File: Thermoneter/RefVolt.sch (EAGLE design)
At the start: 4 parts, among them IC1 OP-AMP-1TSV521ICT

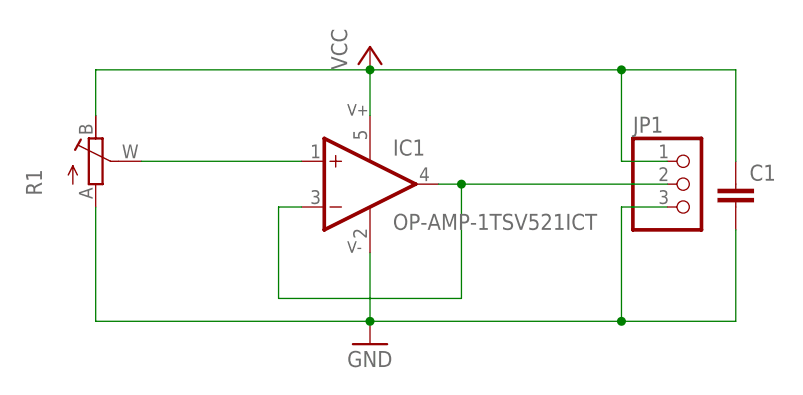
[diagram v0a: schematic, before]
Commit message: _Something
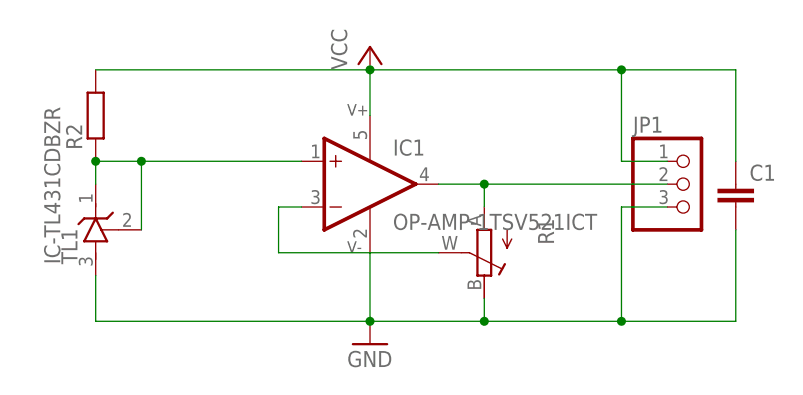
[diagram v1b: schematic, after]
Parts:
- added R2: (no value), Namenlos:R_0805
- added TL1: IC-TL431CDBZR, Namenlos:IC-TL431CDBZR
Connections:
- new net N$7: IC1G$1.+IN, R2.1, TL1.C, TL1.R
- net GND: now also R1.E, TL1.A; no longer R1.A
- net N$1: now also R1.S; no longer IC1G$1.OUT, JP1.2
- net N$4: now also IC1G$1.OUT, JP1.2, R1.A; no longer IC1G$1.+IN, R1.S
- net VCC: now also R2.2; no longer R1.E
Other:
- moved on the sheet: R1
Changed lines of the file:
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@@
 <?xml version="1.0" encoding="utf-8"?>
 <!DOCTYPE eagle SYSTEM "eagle.dtd">
-<eagle version="8.0.0">
+<eagle version="8.0.1">
 <drawing>
 <settings>
@@
 <part name="GND1" library="supply1" deviceset="GND" device=""/>
 <part name="P+1" library="supply1" deviceset="VCC" device=""/>
+<part name="TL1" library="Namenlos" deviceset="IC-TL431" device="CDBZR"/>
+<part name="R2" library="Namenlos" deviceset="R_" device="0805"/>
 </parts>
 <sheets>
@@
 <instances>
 <instance part="IC1" gate="G$1" x="30.48" y="33.02"/>
-<instance part="R1" gate="G$1" x="0" y="35.56"/>
+<instance part="R1" gate="G$1" x="43.18" y="25.4" rot="R180"/>
 <instance part="IC1" gate="G$2" x="30.48" y="33.02"/>
 <instance part="JP1" gate="A" x="66.04" y="33.02"/>
@@
 <instance part="GND1" gate="1" x="30.48" y="15.24"/>
 <instance part="P+1" gate="VCC" x="30.48" y="48.26"/>
+<instance part="TL1" gate="G$1" x="0" y="27.94" rot="MR90"/>
+<instance part="R2" gate="G$1" x="0" y="40.64" rot="R90"/>
 </instances>
 <busses>
@@
 <pinref part="IC1" gate="G$1" pin="-IN"/>
 <wire x1="22.86" y1="30.48" x2="20.32" y2="30.48" width="0.1524" layer="91"/>
-<wire x1="20.32" y1="30.48" x2="20.32" y2="20.32" width="0.1524" layer="91"/>
-<wire x1="20.32" y1="20.32" x2="40.64" y2="20.32" width="0.1524" layer="91"/>
-<wire x1="40.64" y1="20.32" x2="40.64" y2="33.02" width="0.1524" layer="91"/>
-<pinref part="IC1" gate="G$1" pin="OUT"/>
-<wire x1="40.64" y1="33.02" x2="38.1" y2="33.02" width="0.1524" layer="91"/>
-<pinref part="JP1" gate="A" pin="2"/>
-<wire x1="63.5" y1="33.02" x2="40.64" y2="33.02" width="0.1524" layer="91"/>
-<junction x="40.64" y="33.02"/>
-</segment>
-</net>
-<net name="N$4" class="0">
-<segment>
 <pinref part="R1" gate="G$1" pin="S"/>
-<pinref part="IC1" gate="G$1" pin="+IN"/>
-<wire x1="5.08" y1="35.56" x2="22.86" y2="35.56" width="0.1524" layer="91"/>
+<wire x1="38.1" y1="25.4" x2="20.32" y2="25.4" width="0.1524" layer="91"/>
+<wire x1="20.32" y1="25.4" x2="20.32" y2="30.48" width="0.1524" layer="91"/>
 </segment>
 </net>
@@
 <pinref part="IC1" gate="G$2" pin="V-"/>
 <wire x1="30.48" y1="25.4" x2="30.48" y2="17.78" width="0.1524" layer="91"/>
-<wire x1="30.48" y1="17.78" x2="58.42" y2="17.78" width="0.1524" layer="91"/>
+<wire x1="30.48" y1="17.78" x2="43.18" y2="17.78" width="0.1524" layer="91"/>
+<wire x1="43.18" y1="17.78" x2="58.42" y2="17.78" width="0.1524" layer="91"/>
 <wire x1="58.42" y1="17.78" x2="58.42" y2="30.48" width="0.1524" layer="91"/>
 <pinref part="JP1" gate="A" pin="3"/>
 <wire x1="58.42" y1="30.48" x2="63.5" y2="30.48" width="0.1524" layer="91"/>
-<pinref part="R1" gate="G$1" pin="A"/>
-<wire x1="0" y1="30.48" x2="0" y2="17.78" width="0.1524" layer="91"/>
 <wire x1="0" y1="17.78" x2="30.48" y2="17.78" width="0.1524" layer="91"/>
 <junction x="30.48" y="17.78"/>
@@
 <junction x="58.42" y="17.78"/>
 <pinref part="GND1" gate="1" pin="GND"/>
+<pinref part="R1" gate="G$1" pin="E"/>
+<wire x1="43.18" y1="20.32" x2="43.18" y2="17.78" width="0.1524" layer="91"/>
+<junction x="43.18" y="17.78"/>
+<pinref part="TL1" gate="G$1" pin="A"/>
+<wire x1="0" y1="22.86" x2="0" y2="17.78" width="0.1524" layer="91"/>
 </segment>
 </net>
@@
 <pinref part="JP1" gate="A" pin="1"/>
 <wire x1="58.42" y1="35.56" x2="63.5" y2="35.56" width="0.1524" layer="91"/>
-<pinref part="R1" gate="G$1" pin="E"/>
-<wire x1="0" y1="40.64" x2="0" y2="45.72" width="0.1524" layer="91"/>
 <wire x1="0" y1="45.72" x2="30.48" y2="45.72" width="0.1524" layer="91"/>
 <junction x="30.48" y="45.72"/>
@@
 <junction x="58.42" y="45.72"/>
 <pinref part="P+1" gate="VCC" pin="VCC"/>
-</segment>
-</net>
+<pinref part="R2" gate="G$1" pin="2"/>
+</segment>
+</net>
+<net name="N$4" class="0">
+<segment>
+<pinref part="R1" gate="G$1" pin="A"/>
+<pinref part="IC1" gate="G$1" pin="OUT"/>
+<wire x1="43.18" y1="30.48" x2="43.18" y2="33.02" width="0.1524" layer="91"/>
+<wire x1="43.18" y1="33.02" x2="38.1" y2="33.02" width="0.1524" layer="91"/>
+<pinref part="JP1" gate="A" pin="2"/>
+<wire x1="63.5" y1="33.02" x2="43.18" y2="33.02" width="0.1524" layer="91"/>
+<junction x="43.18" y="33.02"/>
+</segment>
+</net>
+<net name="N$7" class="0">
+<segment>
+<pinref part="TL1" gate="G$1" pin="C"/>
+<pinref part="R2" gate="G$1" pin="1"/>
+<pinref part="TL1" gate="G$1" pin="R"/>
+<wire x1="5.08" y1="27.94" x2="5.08" y2="35.56" width="0.1524" layer="91"/>
+<wire x1="5.08" y1="35.56" x2="0" y2="35.56" width="0.1524" layer="91"/>
+<junction x="0" y="35.56"/>
+<wire x1="0" y1="35.56" x2="0" y2="33.02" width="0.1524" layer="91"/>
+<pinref part="IC1" gate="G$1" pin="+IN"/>
+<wire x1="22.86" y1="35.56" x2="5.08" y2="35.56" width="0.1524" layer="91"/>
+<junction x="5.08" y="35.56"/>
+</segment>
+</net>
